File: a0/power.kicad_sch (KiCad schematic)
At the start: 28 parts, among them J4 ESP32 USB, J5 SIM7080G USBC, J6 Conn_01x02, J7 Beagle P9, J8 Beagle P8, U6 AMS1117-3.3

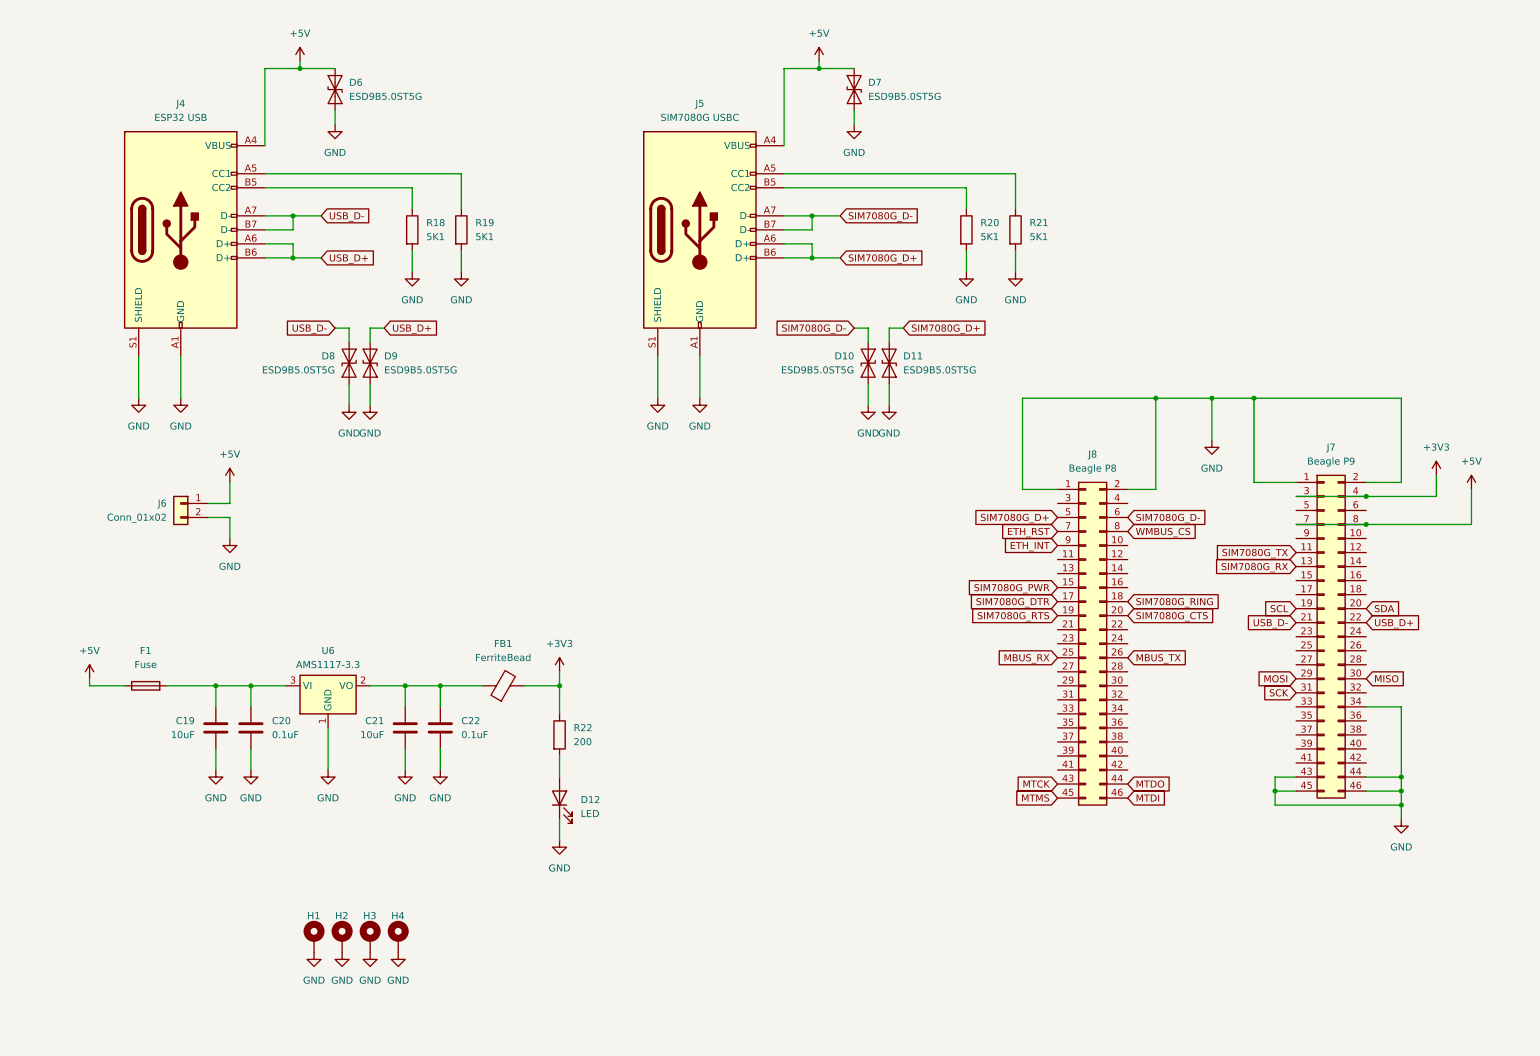
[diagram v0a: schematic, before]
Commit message: update A0
Signed-off-by: Rodney Osodo <socials@rodneyosodo.com>
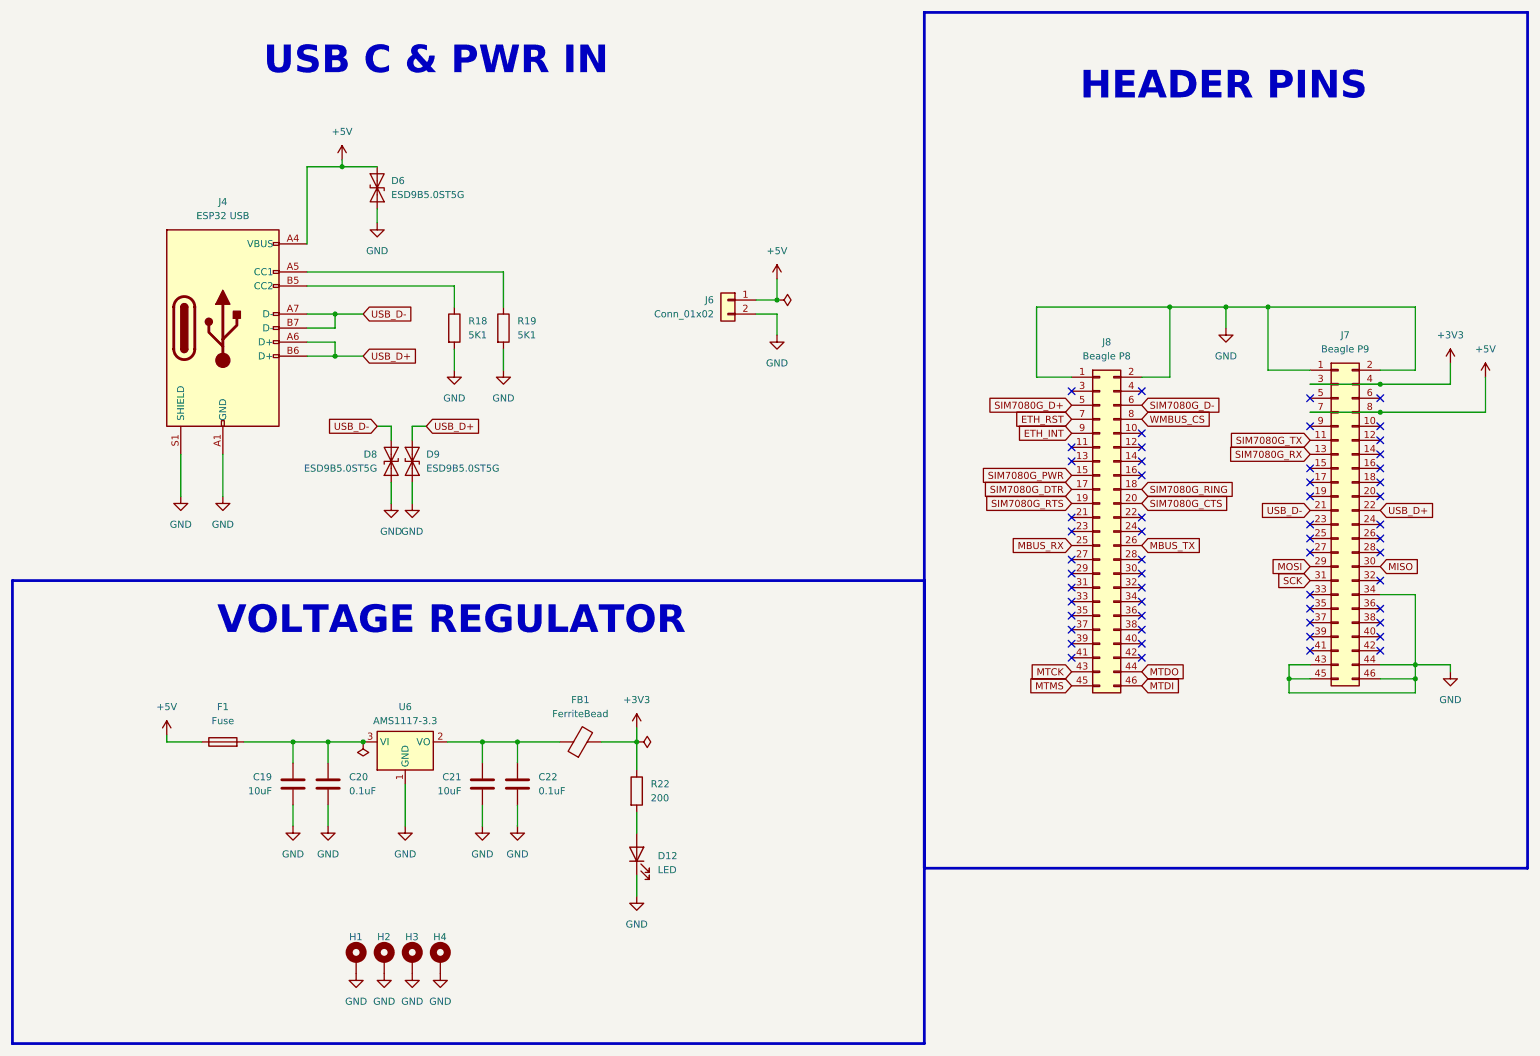
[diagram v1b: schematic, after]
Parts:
- removed D10, D11, D7: ESD9B5.0ST5G, Diode_SMD:D_SOD-923, symbol Diode:ESD9B5.0ST5G
- removed J5: SIM7080G USBC, Connector_USB:USB_C_Receptacle_G-Switch_GT-USB-7010ASV, symbol Connector:USB_C_Receptacle_USB2.0_14P
- removed R20, R21: 5K1, Resistor_SMD:R_0805_2012Metric, symbol Device:R
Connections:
- net SCL: no longer names the net of J7.19 (Pin_19)
- net SDA: no longer names the net of J7.20 (Pin_20)
- no-connect marks 0 -> 56
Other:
- note added: "HEADER PINS"
- note added: "USB C & PWR IN"
- note added: "VOLTAGE REGULATOR"
- company: (none) -> Abstract Machines
- title: (none) -> A0
- moved on the sheet: C19, C20, C21, C22, D12, D6, D8, D9, F1, FB1, H1, H2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

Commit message: fix(A0): update to use modules
Signed-off-by: Rodney Osodo <socials@rodneyosodo.com>
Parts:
- removed C19, C21: 10uF, Capacitor_SMD:C_0805_2012Metric, symbol Device:C
- removed C20, C22: 0.1uF, Capacitor_SMD:C_0805_2012Metric, symbol Device:C
- removed D12: LED, LED_SMD:LED_0805_2012Metric, symbol Device:LED
- removed J6: Conn_01x02, Connector_JST:JST_EH_B2B-EH-A_1x02_P2.50mm_Vertical, symbol Connector_Generic:Conn_01x02
- removed J7: Beagle P9, Connector_PinHeader_2.54mm:PinHeader_2x23_P2.54mm_Vertical, symbol Connector_Generic:Conn_02x23_Odd_Even
- removed J8: Beagle P8, Connector_PinHeader_2.54mm:PinHeader_2x23_P2.54mm_Vertical, symbol Connector_Generic:Conn_02x23_Odd_Even
- removed R22: 200, Resistor_SMD:R_0805_2012Metric, symbol Device:R
- removed U6: AMS1117-3.3, Package_TO_SOT_SMD:SOT-223-3_TabPin2, symbol Regulator_Linear:AMS1117-3.3
- added C10, C11: 0.1uF, Capacitor_SMD:C_0805_2012Metric, symbol Device:C
- added C12, C13, C8, C9: 10uF, Capacitor_SMD:C_0805_2012Metric, symbol Device:C
- added C14: 330uF, Capacitor_SMD:C_Elec_8x10.2, symbol Device:C
- added C5, C6, C7: 4.7uF, Capacitor_SMD:C_0805_2012Metric_Pad1.18x1.45mm_HandSolder, symbol Device:C
- added D1, D7, D8, D9: 40V 3A 550mV@3A Schottky, Diode_SMD:D_SMA-SMB_Universal_Handsoldering, symbol Device:D
- added D10, D6: LED, LED_SMD:LED_0603_1608Metric, symbol Device:LED
- added D5: BZV55C27, Diode_SMD:D_SMA, symbol Diode:BZV55C27
- added J8: Screw_Terminal_01x02, TerminalBlock:TerminalBlock_MaiXu_MX126-5.0-02P_1x02_P5.00mm, symbol Connector:Screw_Terminal_01x02
- added J9: BAT_JST_01x02, Connector_JST:JST_EH_B2B-EH-A_1x02_P2.50mm_Vertical, symbol Connector:Screw_Terminal_01x02
- added L1: 47uH/2A, Inductor_SMD:L_Chilisin_BMRB00060624, symbol Device:L_Ferrite
- added R10: 10k, Resistor_SMD:R_0805_2012Metric_Pad1.20x1.40mm_HandSolder, symbol Device:R
- added R11: 220, Resistor_SMD:R_0603_1608Metric, symbol Device:R
- added R8: 2k, Resistor_SMD:R_0805_2012Metric_Pad1.20x1.40mm_HandSolder, symbol Device:R
- added R9: 220, Resistor_SMD:R_0805_2012Metric_Pad1.20x1.40mm_HandSolder, symbol Device:R
- added TP1, TP2, TP3, TP4: TestPoint, TestPoint:TestPoint_Pad_D1.0mm, symbol Connector:TestPoint
- added U5: MCP73831-2-OT, Package_TO_SOT_SMD:SOT-23-5, symbol Battery_Management:MCP73831-2-OT
- added U6: XL1509-5.0, Package_SO:SOIC-8_3.9x4.9mm_P1.27mm, symbol Regulator_Switching:XL1509-5.0
- added U7, U8: AMS1117-3.3, Package_TO_SOT_SMD:SOT-223-3_TabPin2, symbol Regulator_Linear:AMS1117-3.3
- F1: footprint Fuse:Fuse_1206_3216Metric_Pad1.42x1.75mm_HandSolder -> Fuse:Fuse_1206_3216Metric
- renumbered D6 to D2, D8 to D3, D9 to D4, J4 to J7, R18 to R6, R19 to R7
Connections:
- net +3V3: now also D10.2 (A)
- net +5V: now also C14.1, C5.1, D6.2 (A), D8.2 (A), L1.2, R10.2, U5.4 (V_{DD}), U6.3 (FB); no longer F1.1
- net GND: now also C10.2, C11.2, C12.2, C13.2, C14.2, C5.2, C6.2, C7.2, C8.2, C9.2, D5.2 (A), D9.2 (A), J8.2 (Pin_2), J9.2 (Pin_2), R10.1, R11.2, R8.1, U5.2 (V_{SS}), U6.4 (~{EN}), U6.5 (GND), U6.6 (GND), U6.7 (GND), U6.8 (GND), U7.1 (GND), U8.1 (GND)
- net at FB1.1: now also C12.1, C13.1, TP4.1, U7.2 (VO), U8.2 (VO)
- net at F1.2: now also C10.1, C11.1, C9.1, U7.3 (VI), U8.3 (VI)
- new net: D6.1 (K), R9.1
- new net: D9.1 (K), L1.1, U6.2 (OUT)
- new net: D7.1 (K), D8.1 (K), F1.1, TP3.1
- new net: R8.2, U5.5 (PROG)
- new net: D10.1 (K), R11.1
- new net: D1.2 (A), J8.1 (Pin_1)
- new net: R9.2, U5.1 (STAT)
- new net VBAT: C6.1, C7.1, D7.2 (A), J9.1 (Pin_1), TP2.1, U5.3 (V_{BAT})
- new net VIN: C8.1, D1.1 (K), D5.1 (K), TP1.1, U6.1 (VIN)
- no-connect marks 56 -> 0
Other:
- note added: "5V - 3.3V CONV"
- note added: "BATTERY"
- note added: "BATTERY CHARGER"
- note added: "CURRENT REGULATION SET Fast charge current regulation can be scaled by placing a programming resistor (RPROG) from the PROG input to VSS. The program resistor and the charge current are calculated using the following equation: Ireg = 1000V/Rprog where: Rprog is in kOhms Ireg is charging current in milliamps. Ireg = 1000V/2 = 500mA"
- note added: "Max 24V"
- note added: "Max 3.7V (1 LiPo Battery)"
- note added: "Max 37V"
- note added: "REVERSE POLARITY PROTECTION"
- note added: "Reverse Polarity Protection"
- note added: "VIN - 5V CONV"
- note added: "n - 82%"
- note removed: "HEADER PINS"
- note removed: "VOLTAGE REGULATOR"
- moved on the sheet: D2, D3, D4, FB1, H1, H2, H3, H4, J7, R6, R7
